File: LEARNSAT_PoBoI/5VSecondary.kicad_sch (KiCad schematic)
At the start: 17 parts, among them Q1301 SI7164DP-T1-GE3, Q1302 SI5418DU-T1-GE3, U1301 INA219AIDCNR, U1302 LTC4231IUD-2#TRPBF

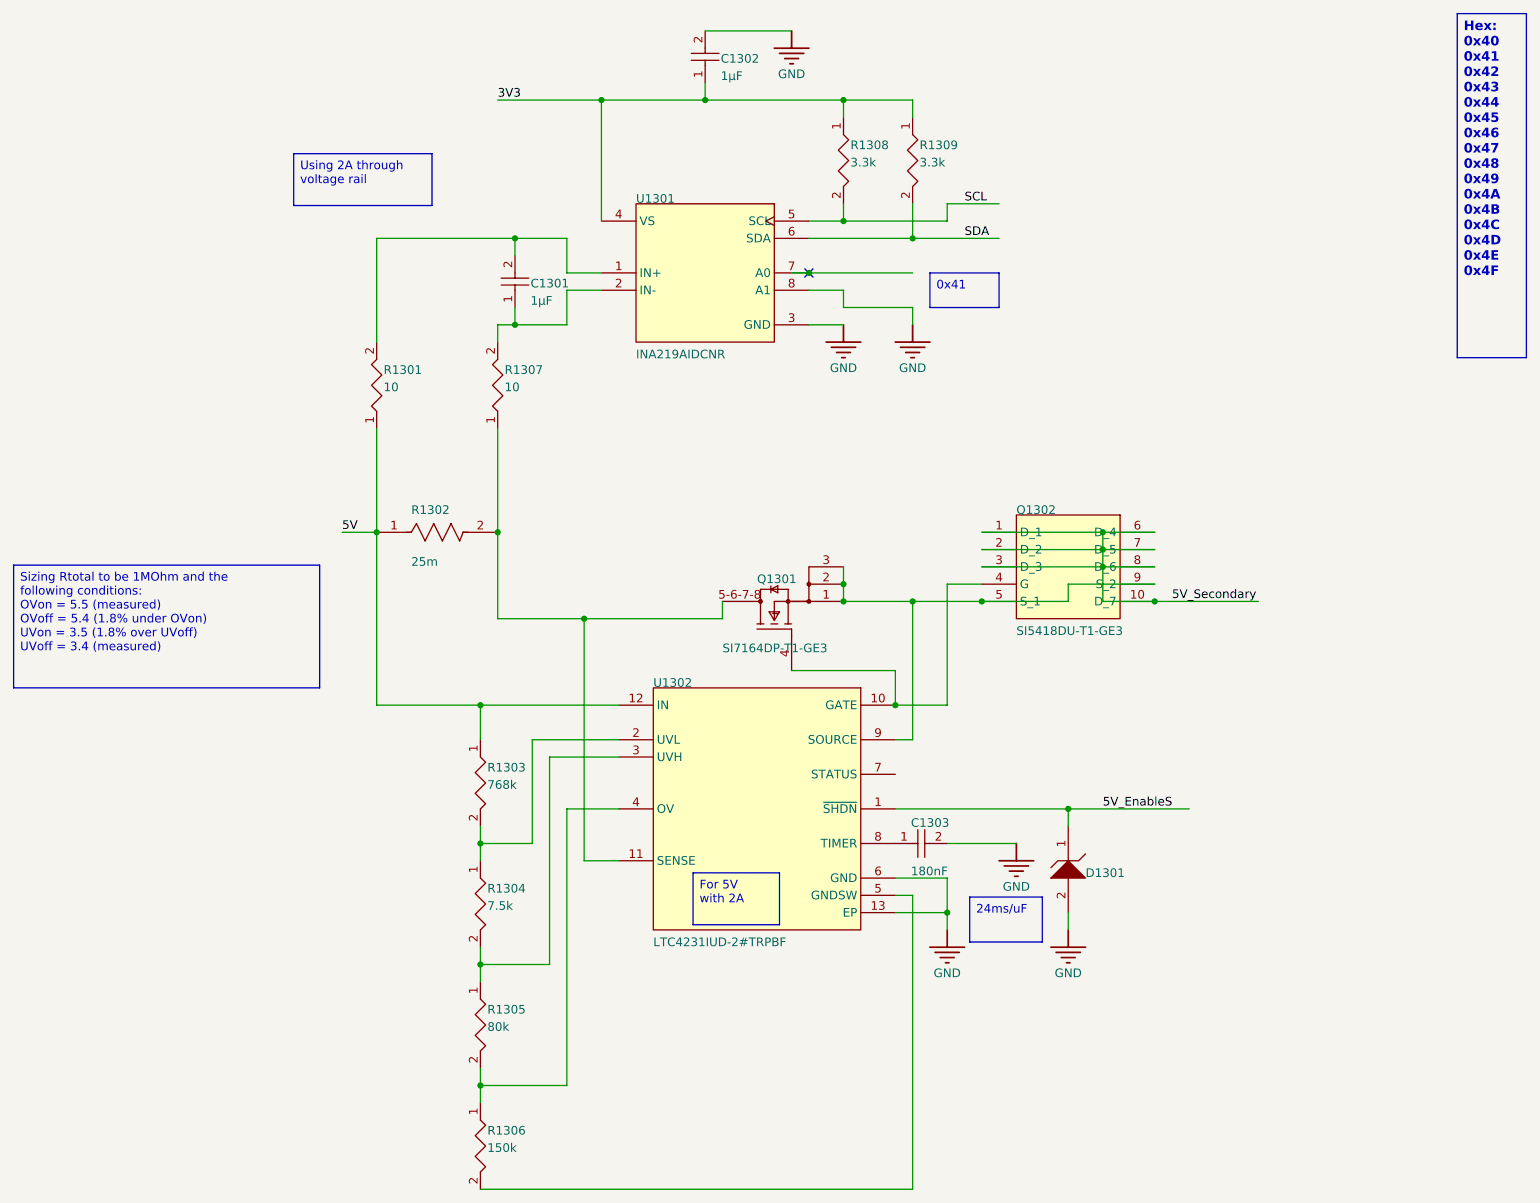
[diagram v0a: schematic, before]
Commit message: Add files via upload
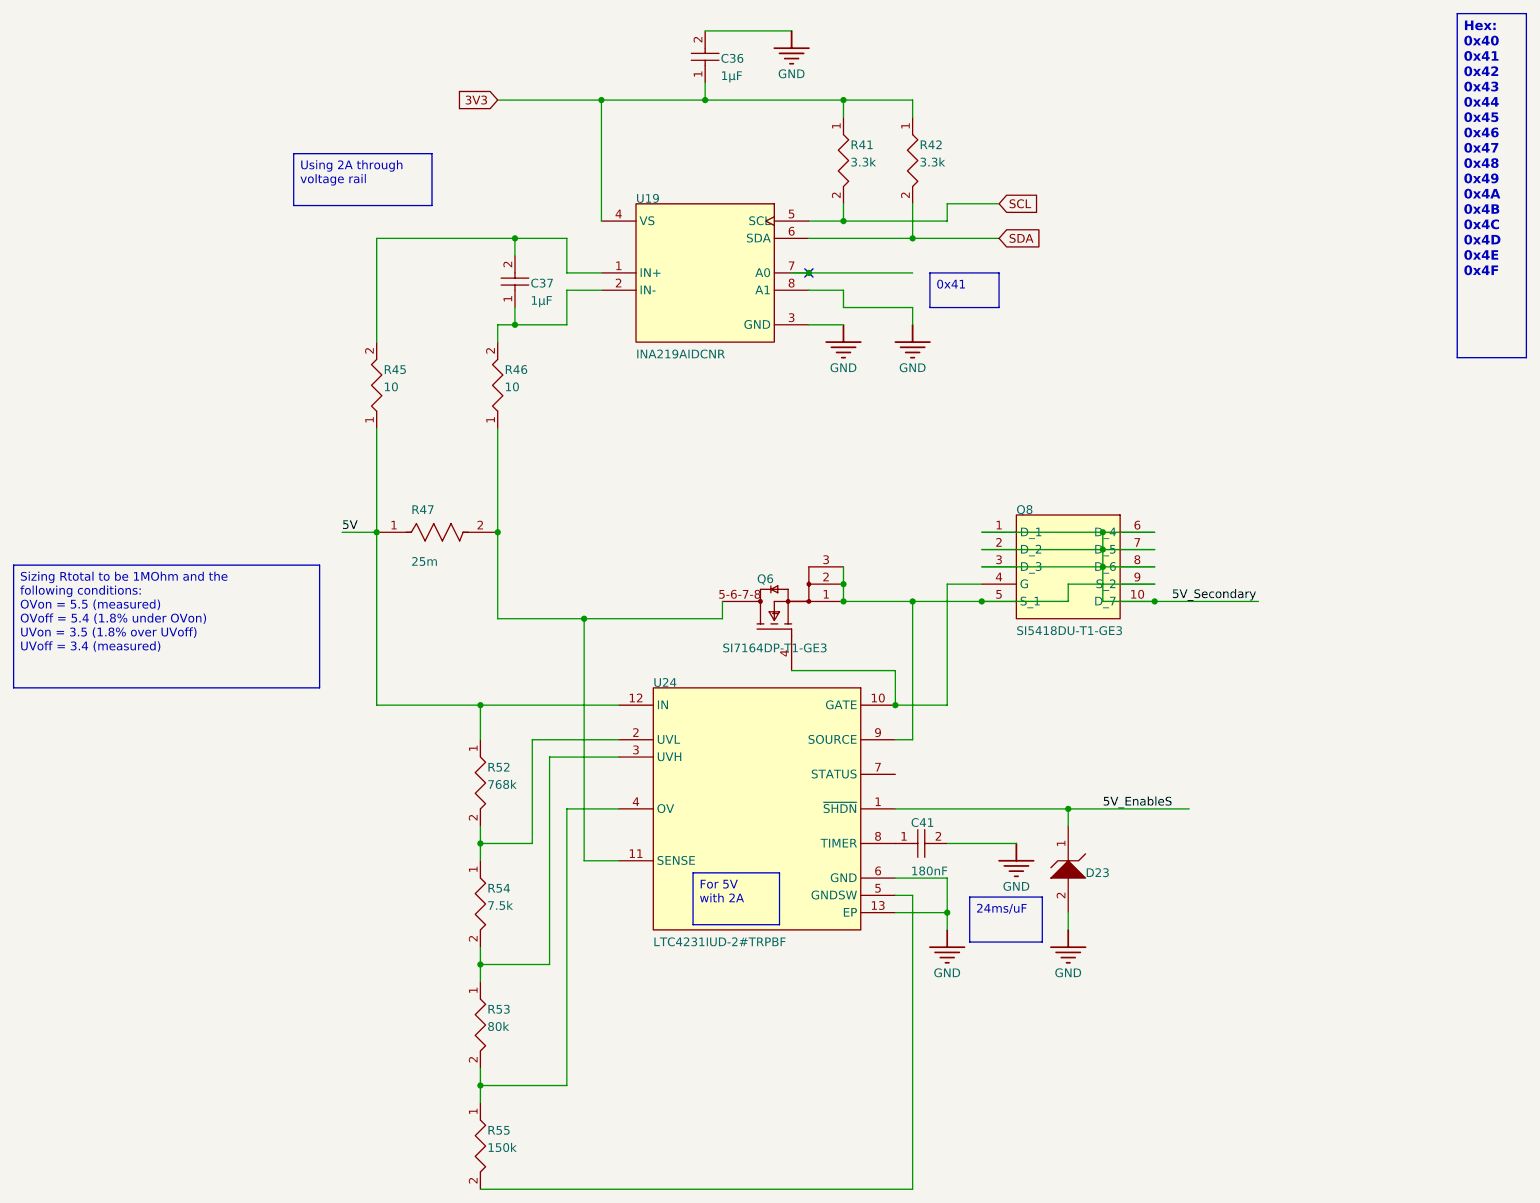
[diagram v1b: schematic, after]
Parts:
- C36: renamed from C1302; footprint Capacitor_SMD:C_0603_1608Metric -> CAPC1608X90X35ML15T15
- C37: renamed from C1301; footprint Capacitor_SMD:C_0603_1608Metric -> CAPC1608X90X40LL10T20
- C41: renamed from C1303; footprint Capacitor_SMD:C_0805_2012Metric -> FP-C0805C-DN-IPC_A
- D23: renamed from D1301; footprint Diode_SMD:D_SOD-323 -> ONSC-SOD-323-2-477-02_V
- Q6: renamed from Q1301; footprint Package_SO:Vishay_PowerPAK_1212-8_Single -> Vishay_S17-0173-SINGLE_MFG
- Q8: renamed from Q1302; footprint Package_SO:Vishay_PowerPAK_1212-8_Single -> SI5418DU-T1-GE3-Footprint-1
- R41: renamed from R1308; footprint Resistor_SMD:R_1210_3225Metric -> FP-CRCW1210-e3-IPC_C
- R42: renamed from R1309; footprint Resistor_SMD:R_1210_3225Metric -> FP-CRCW1210-e3-IPC_C
- R45: renamed from R1301; footprint Resistor_SMD:R_0402_1005Metric -> RESC0402(1005)_L
- R46: renamed from R1307; footprint Resistor_SMD:R_0402_1005Metric -> RESC0402(1005)_L
- R47: renamed from R1302; footprint Resistor_SMD:R_1206_3216Metric -> FP-CSR1206-IPC_C
- R52: renamed from R1303; footprint Resistor_SMD:R_0402_1005Metric -> RESC0402(1005)_L
- R53: renamed from R1305; footprint Resistor_SMD:R_0603_1608Metric -> FP-PTN0603-IPC_B
- R54: renamed from R1304; footprint Resistor_SMD:R_1206_3216Metric -> FP-CRCW1206-e3-IPC_A
- R55: renamed from R1306; footprint Resistor_SMD:R_1206_3216Metric -> FP-RT1206-IPC_C
- U19: renamed from U1301; footprint INA219AIDCNR:SOT65P280X145-8N -> FP-DCN0008A-IPC_A
- U24: renamed from U1302; footprint LTC4231IUD-2_TRPBF:QFN50P300X300X80-13N -> FP-UD-12-05-08-1855-IPC_A
